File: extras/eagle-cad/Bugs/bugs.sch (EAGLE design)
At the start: 19 parts, among them M1 WIREPADSMD5-2,5, M2 WIREPADSMD5-2,5, M3 WIREPADSMD5-2,5, M4 WIREPADSMD5-2,5

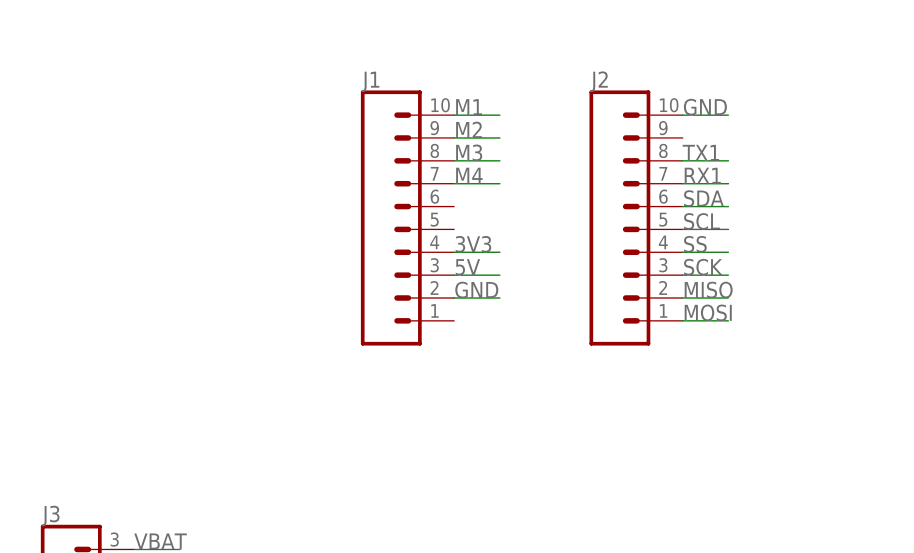
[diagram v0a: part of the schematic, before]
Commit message: Cleanup
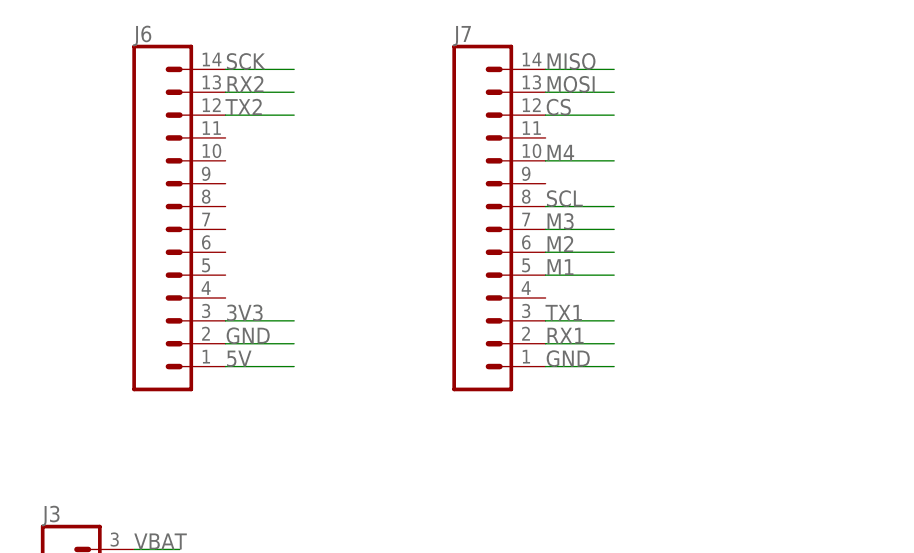
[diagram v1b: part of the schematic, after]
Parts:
- removed J1, J2: (no value), SparkFun-Connectors:CONN_10NO_SILK_PTH_FEMALE
- added J6, J7: (no value), SparkFun-Connectors:CONN_14NO_SILK
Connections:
- removed net SS: J2.4
- new net CS: J7.12
- new net RX2: J6.13
- new net TX2: J6.12
- net 3V3: now also J6.3; no longer J1.4
- net 5V: now also J6.1; no longer J1.3
- net GND: now also J6.2, J7.1; no longer J1.2, J2.10
- net M1: now also J7.5; no longer J1.10
- net M2: now also J7.6; no longer J1.9
- net M3: now also J7.7; no longer J1.8
- net M4: now also J7.10; no longer J1.7
- net MISO: now also J7.14; no longer J2.2
- net MOSI: now also J7.13; no longer J2.1
- net RX1: now also J7.2; no longer J2.7
- net SCK: now also J6.14; no longer J2.3
- net SCL: now also J7.8; no longer J2.5
- net SDA: no longer J2.6
- net TX1: now also J7.3; no longer J2.8
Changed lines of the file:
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@@
 <part name="GND" library="wirepad" deviceset="WIREPAD" device="SMD5-2,5"/>
 <part name="VBAT" library="wirepad" deviceset="WIREPAD" device="SMD5-2,5"/>
-<part name="J1" library="SparkFun-Connectors" deviceset="CONN_10" device="NO_SILK_PTH_FEMALE"/>
-<part name="J2" library="SparkFun-Connectors" deviceset="CONN_10" device="NO_SILK_PTH_FEMALE"/>
 <part name="J3" library="SparkFun-Connectors" deviceset="CONN_03" device="1X03_NO_SILK"/>
 <part name="J4" library="SparkFun-Connectors" deviceset="CONN_05" device="NO_SILK"/>
@@
 <part name="VBAT4" library="wirepad" deviceset="WIREPAD" device="SMD5-2,5"/>
 <part name="J5" library="SparkFun-Connectors" deviceset="CONN_03" device="1X03_NO_SILK"/>
+<part name="J6" library="SparkFun-Connectors" deviceset="CONN_14" device="NO_SILK"/>
+<part name="J7" library="SparkFun-Connectors" deviceset="CONN_14" device="NO_SILK"/>
 </parts>
 <sheets>
@@
 </instance>
 <instance part="VBAT" gate="G$1" x="2.54" y="-12.7" smashed="yes"/>
-<instance part="J1" gate="J1" x="-15.24" y="68.58" smashed="yes">
-<attribute name="VALUE" x="-15.24" y="45.974" size="1.778" layer="96" font="vector"/>
-<attribute name="NAME" x="-15.24" y="76.708" size="1.778" layer="95" font="vector"/>
-</instance>
-<instance part="J2" gate="J1" x="10.16" y="68.58" smashed="yes">
-<attribute name="VALUE" x="10.16" y="45.974" size="1.778" layer="96" font="vector"/>
-<attribute name="NAME" x="10.16" y="76.708" size="1.778" layer="95" font="vector"/>
-</instance>
 <instance part="J3" gate="J$1" x="-48.26" y="22.86" smashed="yes">
 <attribute name="VALUE" x="-50.8" y="15.494" size="1.778" layer="96" font="vector"/>
@@
 <attribute name="VALUE" x="-38.1" y="-42.926" size="1.778" layer="96" font="vector"/>
 </instance>
+<instance part="J6" gate="G$1" x="-40.64" y="63.5"/>
+<instance part="J7" gate="G$1" x="-5.08" y="63.5"/>
 </instances>
 <busses>
@@
 <net name="GND" class="0">
 <segment>
-<pinref part="J1" gate="J1" pin="2"/>
-<wire x1="-5.08" y1="53.34" x2="0" y2="53.34" width="0.1524" layer="91"/>
-<label x="-5.08" y="53.34" size="1.778" layer="95"/>
-</segment>
-<segment>
-<pinref part="J2" gate="J1" pin="10"/>
-<wire x1="20.32" y1="73.66" x2="25.4" y2="73.66" width="0.1524" layer="91"/>
-<label x="20.32" y="73.66" size="1.778" layer="95"/>
-</segment>
-<segment>
 <pinref part="J3" gate="J$1" pin="2"/>
 <wire x1="-40.64" y1="22.86" x2="-35.56" y2="22.86" width="0.1524" layer="91"/>
@@
 <label x="-27.94" y="-35.56" size="1.778" layer="95"/>
 </segment>
+<segment>
+<pinref part="J6" gate="G$1" pin="2"/>
+<wire x1="-30.48" y1="48.26" x2="-22.86" y2="48.26" width="0.1524" layer="91"/>
+<label x="-30.48" y="48.26" size="1.778" layer="95"/>
+</segment>
+<segment>
+<pinref part="J7" gate="G$1" pin="1"/>
+<wire x1="5.08" y1="45.72" x2="12.7" y2="45.72" width="0.1524" layer="91"/>
+<label x="5.08" y="45.72" size="1.778" layer="95"/>
+</segment>
 </net>
 <net name="5V" class="0">
-<segment>
-<pinref part="J1" gate="J1" pin="3"/>
-<wire x1="-5.08" y1="55.88" x2="0" y2="55.88" width="0.1524" layer="91"/>
-<label x="-5.08" y="55.88" size="1.778" layer="95"/>
-</segment>
 <segment>
 <pinref part="J3" gate="J$1" pin="1"/>
@@
 <label x="-27.94" y="-38.1" size="1.778" layer="95"/>
 </segment>
+<segment>
+<pinref part="J6" gate="G$1" pin="1"/>
+<wire x1="-30.48" y1="45.72" x2="-22.86" y2="45.72" width="0.1524" layer="91"/>
+<label x="-30.48" y="45.72" size="1.778" layer="95"/>
+</segment>
 </net>
 <net name="3V3" class="0">
-<segment>
-<pinref part="J1" gate="J1" pin="4"/>
-<wire x1="-5.08" y1="58.42" x2="0" y2="58.42" width="0.1524" layer="91"/>
-<label x="-5.08" y="58.42" size="1.778" layer="95"/>
-</segment>
 <segment>
 <pinref part="J4" gate="G$1" pin="4"/>
@@
 <label x="-43.18" y="-5.08" size="1.778" layer="95"/>
 </segment>
+<segment>
+<pinref part="J6" gate="G$1" pin="3"/>
+<wire x1="-30.48" y1="50.8" x2="-22.86" y2="50.8" width="0.1524" layer="91"/>
+<label x="-30.48" y="50.8" size="1.778" layer="95"/>
+</segment>
 </net>
 <net name="M1" class="0">
-<segment>
-<pinref part="J1" gate="J1" pin="10"/>
-<wire x1="-5.08" y1="73.66" x2="0" y2="73.66" width="0.1524" layer="91"/>
-<label x="-5.08" y="73.66" size="1.778" layer="95"/>
-</segment>
 <segment>
 <pinref part="M1" gate="G$1" pin="P"/>
@@
 <label x="7.62" y="-66.04" size="1.778" layer="95"/>
 </segment>
+<segment>
+<pinref part="J7" gate="G$1" pin="5"/>
+<wire x1="5.08" y1="55.88" x2="12.7" y2="55.88" width="0.1524" layer="91"/>
+<label x="5.08" y="55.88" size="1.778" layer="95"/>
+</segment>
 </net>
 <net name="M2" class="0">
-<segment>
-<pinref part="J1" gate="J1" pin="9"/>
-<wire x1="-5.08" y1="71.12" x2="0" y2="71.12" width="0.1524" layer="91"/>
-<label x="-5.08" y="71.12" size="1.778" layer="95"/>
-</segment>
 <segment>
 <pinref part="M2" gate="G$1" pin="P"/>
@@
 <label x="68.58" y="-20.32" size="1.778" layer="95"/>
 </segment>
+<segment>
+<pinref part="J7" gate="G$1" pin="6"/>
+<wire x1="5.08" y1="58.42" x2="12.7" y2="58.42" width="0.1524" layer="91"/>
+<label x="5.08" y="58.42" size="1.778" layer="95"/>
+</segment>
 </net>
 <net name="M3" class="0">
-<segment>
-<pinref part="J1" gate="J1" pin="8"/>
-<wire x1="-5.08" y1="68.58" x2="0" y2="68.58" width="0.1524" layer="91"/>
-<label x="-5.08" y="68.58" size="1.778" layer="95"/>
-</segment>
 <segment>
 <pinref part="M3" gate="G$1" pin="P"/>
@@
 <label x="71.12" y="-66.04" size="1.778" layer="95"/>
 </segment>
+<segment>
+<pinref part="J7" gate="G$1" pin="7"/>
+<wire x1="5.08" y1="60.96" x2="12.7" y2="60.96" width="0.1524" layer="91"/>
+<label x="5.08" y="60.96" size="1.778" layer="95"/>
+</segment>
 </net>
 <net name="M4" class="0">
-<segment>
-<pinref part="J1" gate="J1" pin="7"/>
-<wire x1="-5.08" y1="66.04" x2="0" y2="66.04" width="0.1524" layer="91"/>
-<label x="-5.08" y="66.04" size="1.778" layer="95"/>
-</segment>
 <segment>
 <pinref part="M4" gate="G$1" pin="P"/>
@@
 <label x="5.08" y="-22.86" size="1.778" layer="95"/>
 </segment>
+<segment>
+<pinref part="J7" gate="G$1" pin="10"/>
+<wire x1="5.08" y1="68.58" x2="12.7" y2="68.58" width="0.1524" layer="91"/>
+<label x="5.08" y="68.58" size="1.778" layer="95"/>
+</segment>
 </net>
 <net name="SCL" class="0">
@@
 </segment>
 <segment>
-<pinref part="J2" gate="J1" pin="5"/>
-<wire x1="20.32" y1="60.96" x2="25.4" y2="60.96" width="0.1524" layer="91"/>
-<label x="20.32" y="60.96" size="1.778" layer="95"/>
+<pinref part="J7" gate="G$1" pin="8"/>
+<wire x1="5.08" y1="63.5" x2="12.7" y2="63.5" width="0.1524" layer="91"/>
+<label x="5.08" y="63.5" size="1.778" layer="95"/>
 </segment>
 </net>
@@
 <label x="-43.18" y="-12.7" size="1.778" layer="95"/>
 </segment>
-<segment>
-<pinref part="J2" gate="J1" pin="6"/>
-<wire x1="20.32" y1="63.5" x2="25.4" y2="63.5" width="0.1524" layer="91"/>
-<label x="20.32" y="63.5" size="1.778" layer="95"/>
-</segment>
-</net>
-<net name="SS" class="0">
-<segment>
-<pinref part="J2" gate="J1" pin="4"/>
-<wire x1="20.32" y1="58.42" x2="25.4" y2="58.42" width="0.1524" layer="91"/>
-<label x="20.32" y="58.42" size="1.778" layer="95"/>
-</segment>
 </net>
 <net name="SCK" class="0">
 <segment>
-<pinref part="J2" gate="J1" pin="3"/>
-<wire x1="20.32" y1="55.88" x2="25.4" y2="55.88" width="0.1524" layer="91"/>
-<label x="20.32" y="55.88" size="1.778" layer="95"/>
+<pinref part="J6" gate="G$1" pin="14"/>
+<wire x1="-30.48" y1="78.74" x2="-22.86" y2="78.74" width="0.1524" layer="91"/>
+<label x="-30.48" y="78.74" size="1.778" layer="95"/>
 </segment>
 </net>
 <net name="MISO" class="0">
 <segment>
-<pinref part="J2" gate="J1" pin="2"/>
-<wire x1="20.32" y1="53.34" x2="25.4" y2="53.34" width="0.1524" layer="91"/>
-<label x="20.32" y="53.34" size="1.778" layer="95"/>
+<pinref part="J7" gate="G$1" pin="14"/>
+<wire x1="5.08" y1="78.74" x2="12.7" y2="78.74" width="0.1524" layer="91"/>
+<label x="5.08" y="78.74" size="1.778" layer="95"/>
 </segment>
 </net>
 <net name="MOSI" class="0">
 <segment>
-<pinref part="J2" gate="J1" pin="1"/>
-<wire x1="20.32" y1="50.8" x2="25.4" y2="50.8" width="0.1524" layer="91"/>
-<label x="20.32" y="50.8" size="1.778" layer="95"/>
+<pinref part="J7" gate="G$1" pin="13"/>
+<wire x1="5.08" y1="76.2" x2="12.7" y2="76.2" width="0.1524" layer="91"/>
+<label x="5.08" y="76.2" size="1.778" layer="95"/>
 </segment>
 </net>
@@
 </segment>
 <segment>
-<pinref part="J2" gate="J1" pin="7"/>
-<wire x1="20.32" y1="66.04" x2="25.4" y2="66.04" width="0.1524" layer="91"/>
-<label x="20.32" y="66.04" size="1.778" layer="95"/>
+<pinref part="J7" gate="G$1" pin="2"/>
+<wire x1="5.08" y1="48.26" x2="12.7" y2="48.26" width="0.1524" layer="91"/>
+<label x="5.08" y="48.26" size="1.778" layer="95"/>
 </segment>
 </net>
@@
 <net name="TX1" class="0">
 <segment>
-<pinref part="J2" gate="J1" pin="8"/>
-<wire x1="20.32" y1="68.58" x2="25.4" y2="68.58" width="0.1524" layer="91"/>
-<label x="20.32" y="68.58" size="1.778" layer="95"/>
-</segment>
-</net>
+<pinref part="J7" gate="G$1" pin="3"/>
+<wire x1="5.08" y1="50.8" x2="12.7" y2="50.8" width="0.1524" layer="91"/>
+<label x="5.08" y="50.8" size="1.778" layer="95"/>
+</segment>
+</net>
+<net name="RX2" class="0">
+<segment>
+<pinref part="J6" gate="G$1" pin="13"/>
+<wire x1="-30.48" y1="76.2" x2="-22.86" y2="76.2" width="0.1524" layer="91"/>
+<label x="-30.48" y="76.2" size="1.778" layer="95"/>
+</segment>
+</net>
+<net name="TX2" class="0">
+<segment>
+<pinref part="J6" gate="G$1" pin="12"/>
+<wire x1="-30.48" y1="73.66" x2="-22.86" y2="73.66" width="0.1524" layer="91"/>
+<label x="-30.48" y="73.66" size="1.778" layer="95"/>
+</segment>
+</net>
+<net name="CS" class="0">
+<segment>
+<pinref part="J7" gate="G$1" pin="12"/>
+<wire x1="5.08" y1="73.66" x2="12.7" y2="73.66" width="0.1524" layer="91"/>
+<label x="5.08" y="73.66" size="1.778" layer="95"/>
+</segment>
+</net>
